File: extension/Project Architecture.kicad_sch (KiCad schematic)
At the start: 0 parts

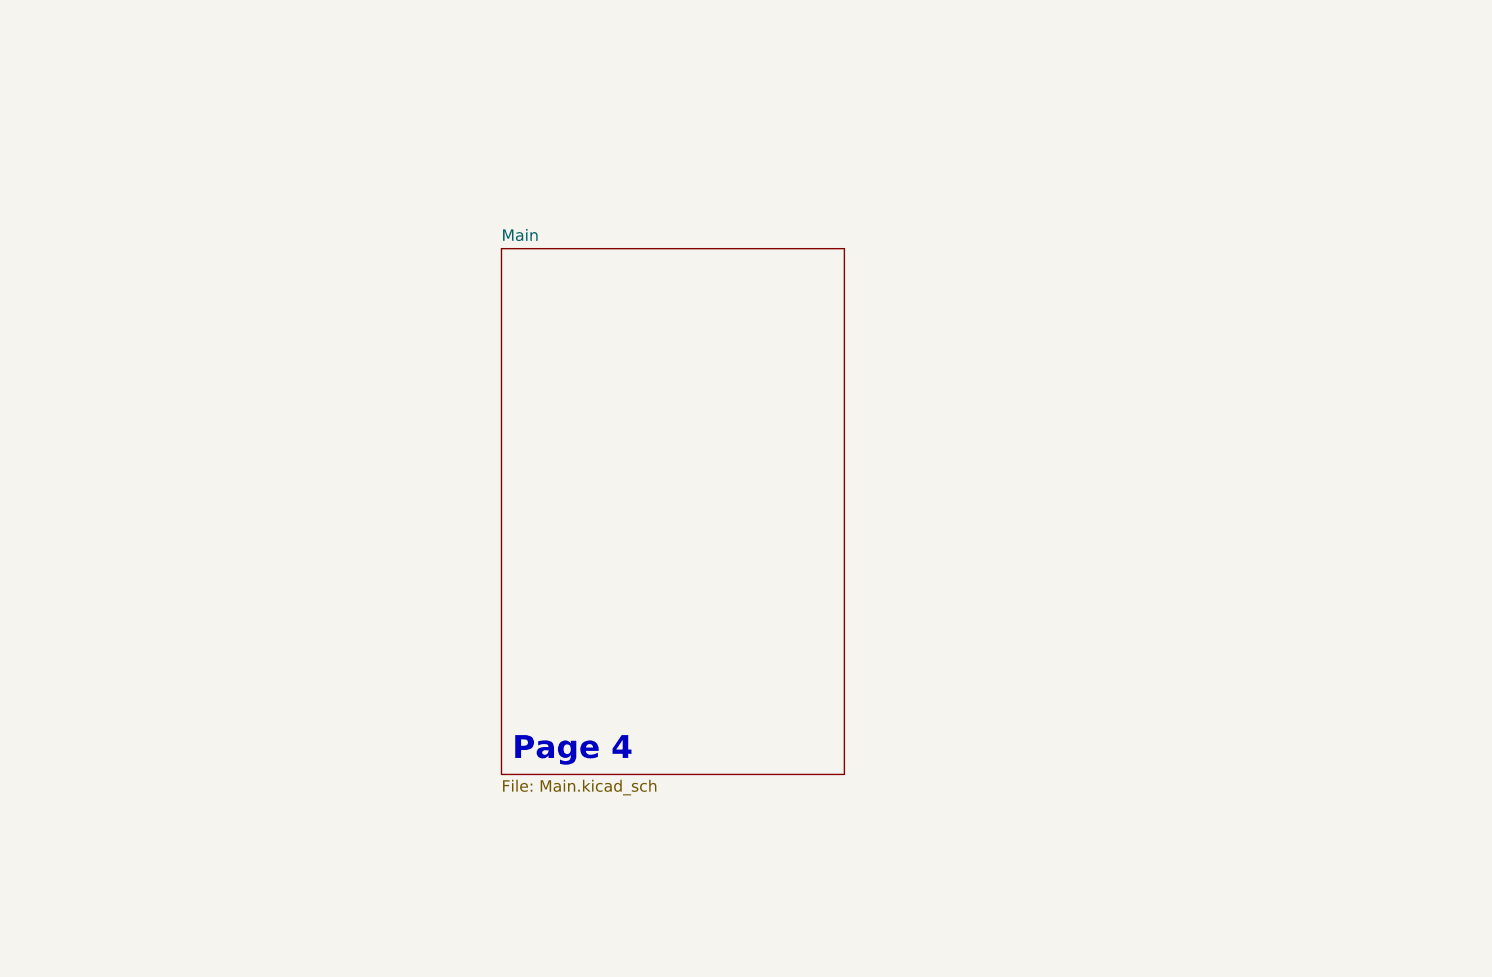
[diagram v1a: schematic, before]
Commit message: First version of the Layout and the Schematics is done
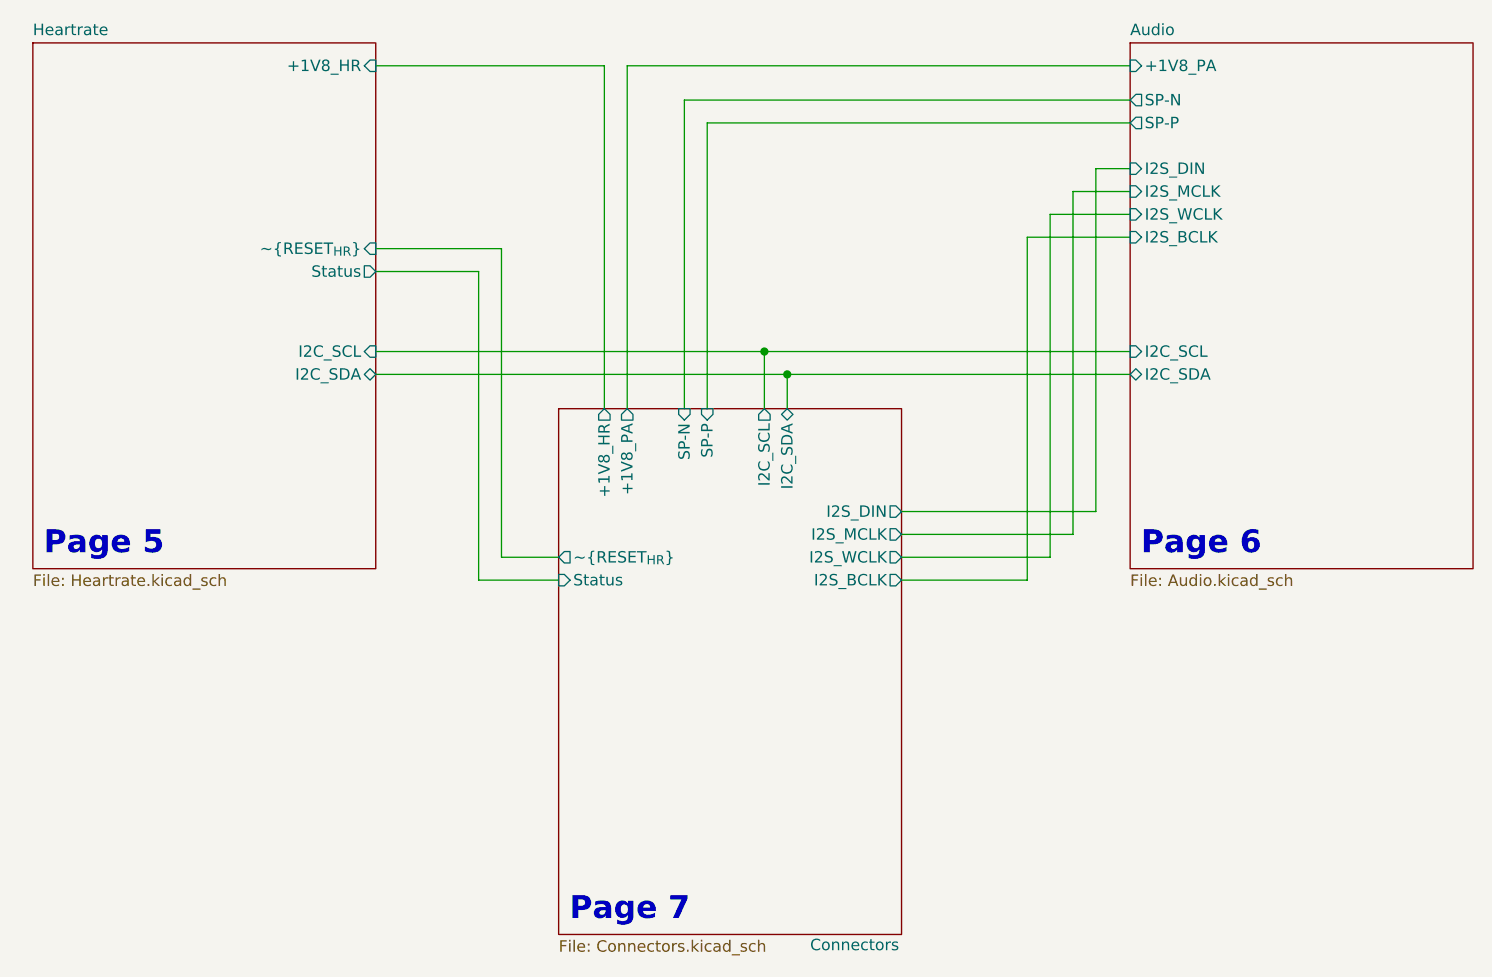
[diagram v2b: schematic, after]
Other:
- sheet Main renamed Heartrate
- added sheet Audio (Audio.kicad_sch)
- added sheet Connectors (Connectors.kicad_sch)
- sheet Heartrate: file Main.kicad_sch -> Heartrate.kicad_sch
- sheet Heartrate ports: added +1V8_HR, I2C_SCL, I2C_SDA, Status, ~{RESET_{HR}}; removed none
- note added: "Page 5"
- note added: "Page 6"
- note added: "Page 7"
- note removed: "Page 4"
